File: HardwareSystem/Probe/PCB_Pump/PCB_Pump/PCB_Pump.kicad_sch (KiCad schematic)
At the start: 4 parts, among them Q1 IRF510

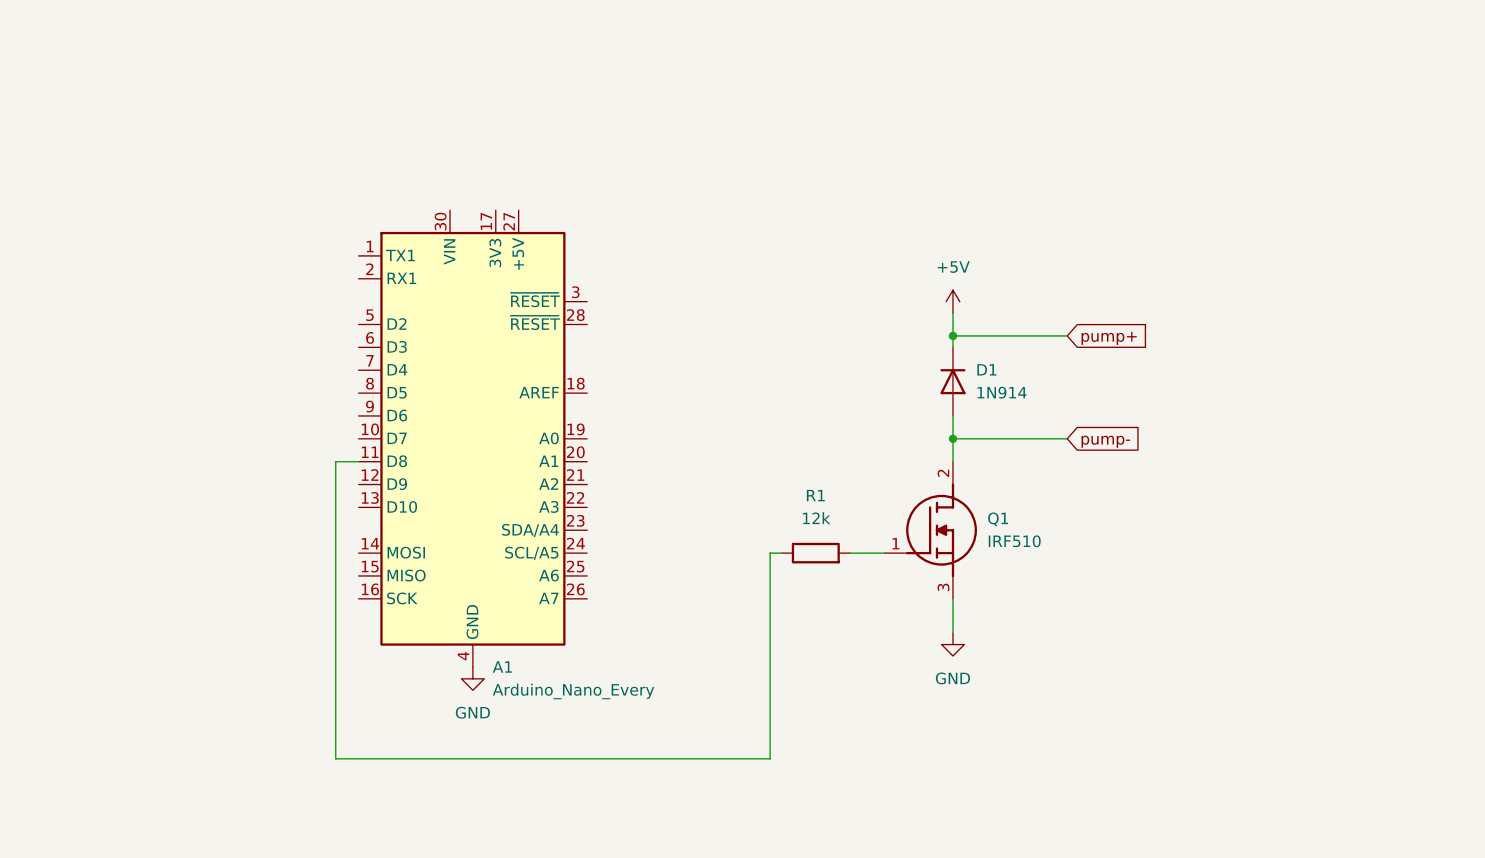
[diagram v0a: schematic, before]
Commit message: pump pcb work
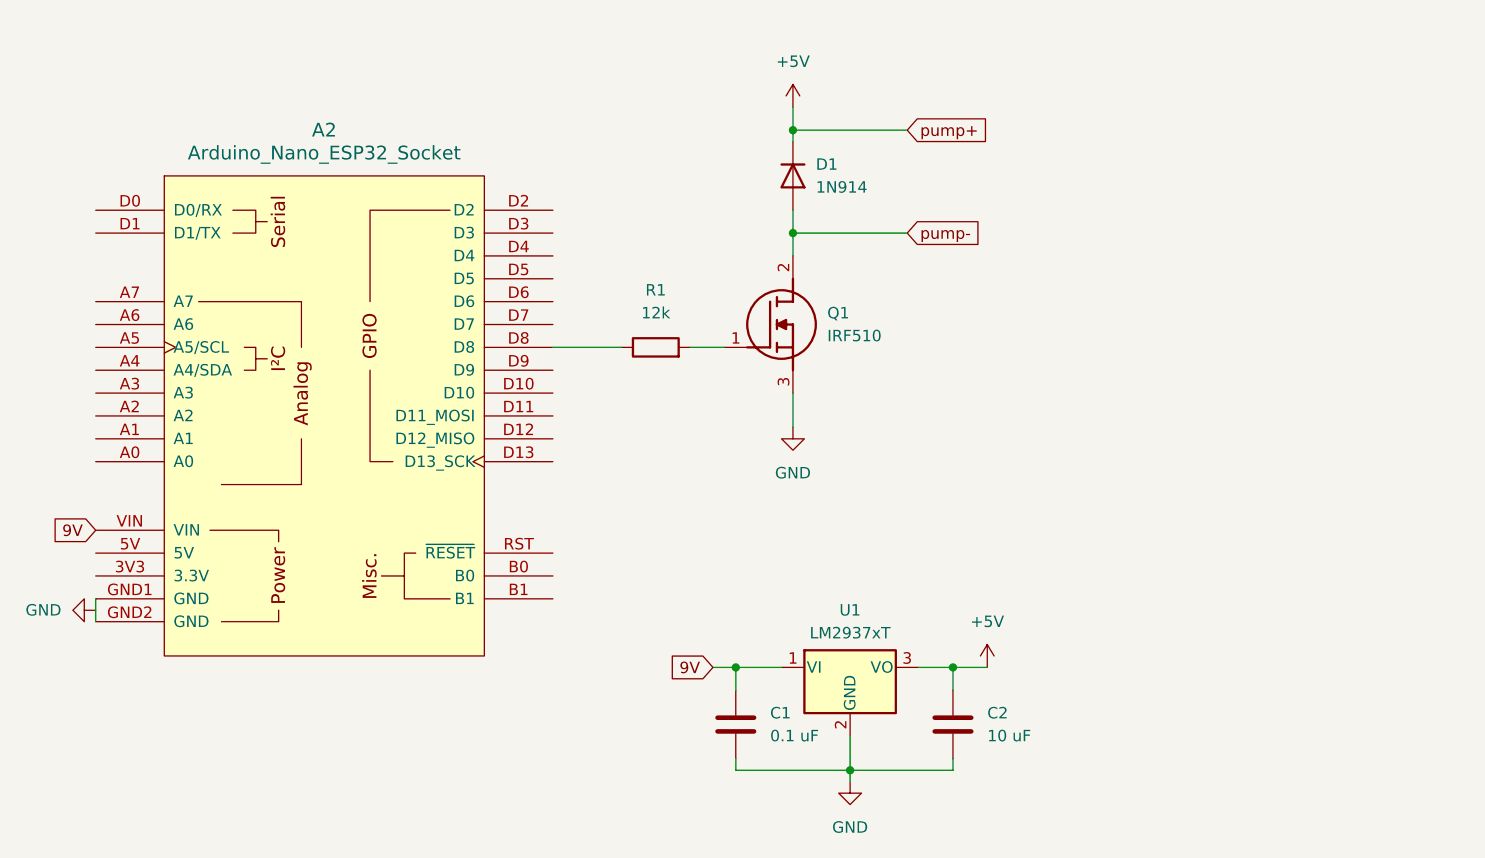
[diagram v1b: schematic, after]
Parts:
- removed A1: Arduino_Nano_Every, Module:Arduino_Nano, symbol MCU_Module:Arduino_Nano_Every
- added A2: Arduino_Nano_ESP32_Socket, footprints:Arduino_Nano_ESP32_Socket, symbol arduino-library:Arduino_Nano_ESP32_Socket
- added C1: 0.1 uF, Capacitor_THT:C_Axial_L3.8mm_D2.6mm_P7.50mm_Horizontal, symbol Device:C
- added C2: 10 uF, Capacitor_THT:C_Axial_L5.1mm_D3.1mm_P7.50mm_Horizontal, symbol Device:C
- added U1: LM2937xT, Package_TO_SOT_THT:TO-220-3_Vertical, symbol Regulator_Linear:LM2937xT
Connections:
- net +5V: now also C2.1, U1.3 (VO)
- net GND: now also C1.2, C2.2, U1.2 (GND)
- net at R1.1: now also A2.D8
- new net: A2.GND1 (GND), A2.GND2 (GND)
- new net 9V: A2.VIN, C1.1, U1.1 (VI)
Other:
- moved on the sheet: D1, Q1, R1

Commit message: finished PCB pump
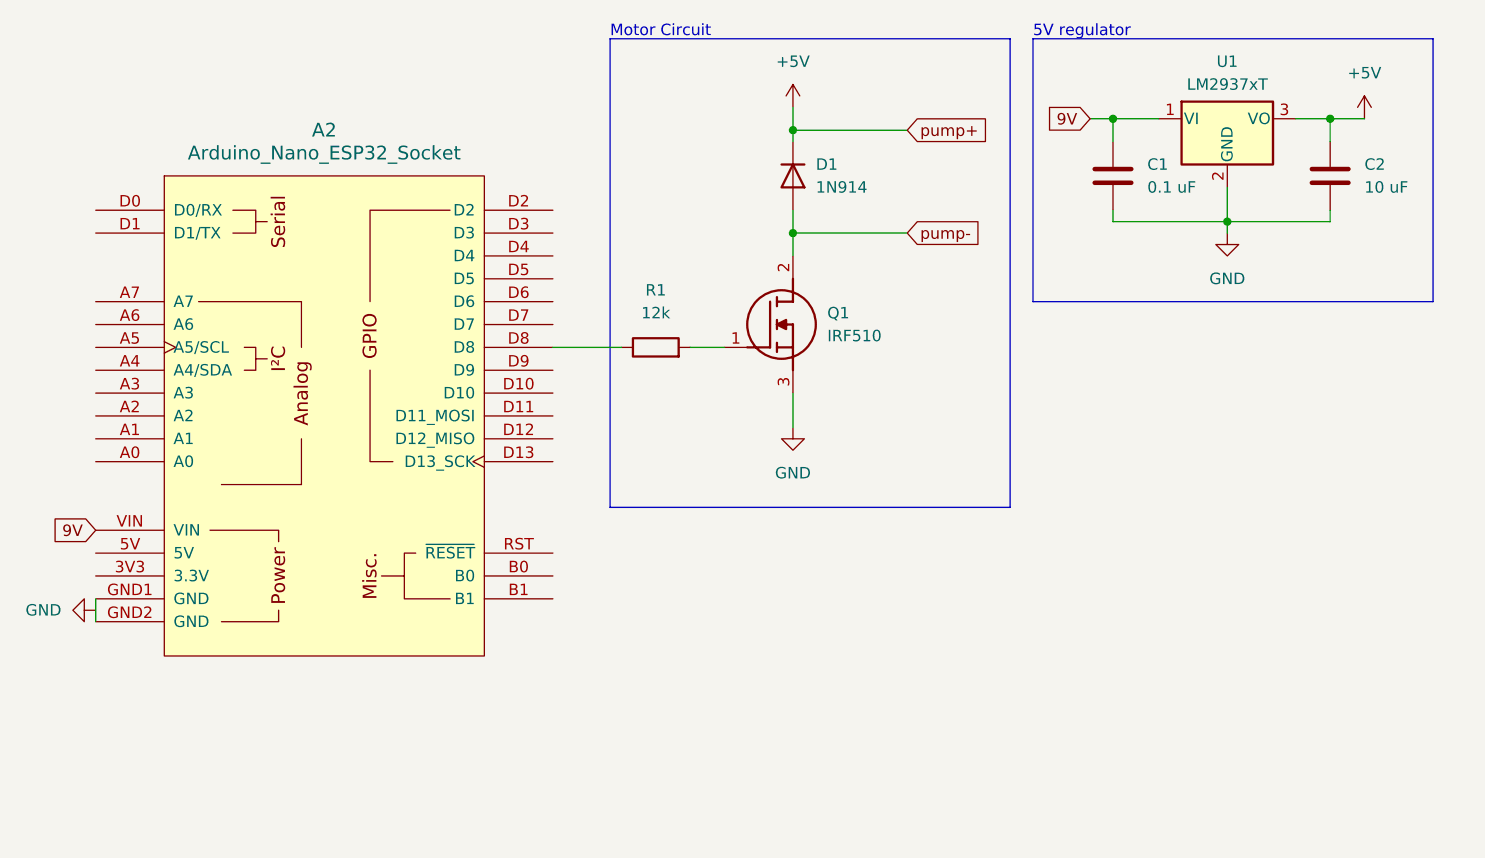
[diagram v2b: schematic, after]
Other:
- note added: "5V regulator"
- note added: "Motor Circuit"
- moved on the sheet: C1, C2, U1
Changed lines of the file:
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@@
 (kicad_sch (version 20230121) (generator eeschema)
   (paper "A4")
-  (junction (at 110.49 104.14) (diameter 0) (color 0 0 0 0)
-  )
-  (junction (at 121.92 92.71) (diameter 0) (color 0 0 0 0)
+  (junction (at 152.4 43.18) (diameter 0) (color 0 0 0 0)
+  )
+  (junction (at 163.83 31.75) (diameter 0) (color 0 0 0 0)
   )
   (junction (at 104.14 44.45) (diameter 0) (color 0 0 0 0)
@@
   (junction (at 104.14 33.02) (diameter 0) (color 0 0 0 0)
   )
-  (junction (at 97.79 92.71) (diameter 0) (color 0 0 0 0)
+  (junction (at 139.7 31.75) (diameter 0) (color 0 0 0 0)
   )
   (wire (pts (xy 104.14 62.23) (xy 104.14 66.04))
@@
     (stroke (width 0) (type default))
   )
-  (wire (pts (xy 95.25 92.71) (xy 97.79 92.71))
-    (stroke (width 0) (type default))
-  )
-  (wire (pts (xy 121.92 92.71) (xy 125.73 92.71))
+  (wire (pts (xy 137.16 31.75) (xy 139.7 31.75))
+    (stroke (width 0) (type default))
+  )
+  (wire (pts (xy 163.83 31.75) (xy 167.64 31.75))
     (stroke (width 0) (type default))
   )
@@
     (stroke (width 0) (type default))
   )
-  (wire (pts (xy 97.79 92.71) (xy 97.79 95.25))
-    (stroke (width 0) (type default))
-  )
-  (wire (pts (xy 110.49 104.14) (xy 121.92 104.14))
-    (stroke (width 0) (type default))
-  )
-  (wire (pts (xy 121.92 102.87) (xy 121.92 104.14))
-    (stroke (width 0) (type default))
-  )
-  (wire (pts (xy 97.79 104.14) (xy 110.49 104.14))
+  (wire (pts (xy 139.7 31.75) (xy 139.7 34.29))
+    (stroke (width 0) (type default))
+  )
+  (wire (pts (xy 152.4 43.18) (xy 163.83 43.18))
+    (stroke (width 0) (type default))
+  )
+  (wire (pts (xy 163.83 41.91) (xy 163.83 43.18))
+    (stroke (width 0) (type default))
+  )
+  (wire (pts (xy 139.7 43.18) (xy 152.4 43.18))
     (stroke (width 0) (type default))
   )
@@
     (stroke (width 0) (type default))
   )
-  (wire (pts (xy 121.92 92.71) (xy 121.92 95.25))
+  (wire (pts (xy 163.83 31.75) (xy 163.83 34.29))
     (stroke (width 0) (type default))
   )
@@
     (stroke (width 0) (type default))
   )
-  (wire (pts (xy 110.49 105.41) (xy 110.49 104.14))
+  (wire (pts (xy 152.4 44.45) (xy 152.4 43.18))
     (stroke (width 0) (type default))
   )
@@
     (stroke (width 0) (type default))
   )
-  (wire (pts (xy 110.49 104.14) (xy 110.49 100.33))
+  (wire (pts (xy 152.4 43.18) (xy 152.4 39.37))
     (stroke (width 0) (type default))
   )
@@
     (stroke (width 0) (type default))
   )
-  (wire (pts (xy 97.79 92.71) (xy 102.87 92.71))
-    (stroke (width 0) (type default))
-  )
-  (wire (pts (xy 97.79 102.87) (xy 97.79 104.14))
-    (stroke (width 0) (type default))
-  )
-  (wire (pts (xy 118.11 92.71) (xy 121.92 92.71))
-    (stroke (width 0) (type default))
-  )
-  (global_label "9V" (shape input) (at 95.25 92.71 180) (fields_autoplaced)
+  (wire (pts (xy 139.7 31.75) (xy 144.78 31.75))
+    (stroke (width 0) (type default))
+  )
+  (wire (pts (xy 139.7 41.91) (xy 139.7 43.18))
+    (stroke (width 0) (type default))
+  )
+  (wire (pts (xy 160.02 31.75) (xy 163.83 31.75))
+    (stroke (width 0) (type default))
+  )
+  (rectangle (start 130.81 22.86) (end 175.26 52.07)
+    (stroke (width 0) (type default))
+    (fill (type none))
+  )
+  (rectangle (start 83.82 22.86) (end 128.27 74.93)
+    (stroke (width 0) (type default))
+    (fill (type none))
+  )
+  (text "5V regulator" (at 130.81 22.86 0)
+    (effects (font (size 1.27 1.27)) (justify left bottom))
+  )
+  (text "Motor Circuit" (at 83.82 22.86 0)
+    (effects (font (size 1.27 1.27)) (justify left bottom))
+  )
+  (global_label "9V" (shape input) (at 137.16 31.75 180) (fields_autoplaced)
     (effects (font (size 1.27 1.27)) (justify right))
-    (property "Intersheetrefs" "${INTERSHEET_REFS}" (at 89.9667 92.71 0)
+    (property "Intersheetrefs" "${INTERSHEET_REFS}" (at 131.8767 31.75 0)
       (effects (font (size 1.27 1.27)) (justify right) hide)
     )
@@
     )
   )
-  (symbol (lib_id "power:GND") (at 110.49 105.41 0) (unit 1)
-    (in_bom yes) (on_board yes) (dnp no) (fields_autoplaced)
-    (property "Reference" "#PWR05" (at 110.49 111.76 0)
-      (effects (font (size 1.27 1.27)) hide)
-    )
-    (property "Value" "GND" (at 110.49 110.49 0)
-      (effects (font (size 1.27 1.27)))
-    )
-    (property "Footprint" "" (at 110.49 105.41 0)
-      (effects (font (size 1.27 1.27)) hide)
-    )
-    (property "Datasheet" "" (at 110.49 105.41 0)
+  (symbol (lib_id "power:GND") (at 152.4 44.45 0) (unit 1)
+    (in_bom yes) (on_board yes) (dnp no) (fields_autoplaced)
+    (property "Reference" "#PWR05" (at 152.4 50.8 0)
+      (effects (font (size 1.27 1.27)) hide)
+    )
+    (property "Value" "GND" (at 152.4 49.53 0)
+      (effects (font (size 1.27 1.27)))
+    )
+    (property "Footprint" "" (at 152.4 44.45 0)
+      (effects (font (size 1.27 1.27)) hide)
+    )
+    (property "Datasheet" "" (at 152.4 44.45 0)
       (effects (font (size 1.27 1.27)) hide)
     )
@@
     )
   )
-  (symbol (lib_id "Regulator_Linear:LM2937xT") (at 110.49 92.71 0) (unit 1)
-    (in_bom yes) (on_board yes) (dnp no) (fields_autoplaced)
-    (property "Reference" "U1" (at 110.49 86.36 0)
-      (effects (font (size 1.27 1.27)))
-    )
-    (property "Value" "LM2937xT" (at 110.49 88.9 0)
-      (effects (font (size 1.27 1.27)))
-    )
-    (property "Footprint" "Package_TO_SOT_THT:TO-220-3_Vertical" (at 110.49 86.995 0)
+  (symbol (lib_id "Regulator_Linear:LM2937xT") (at 152.4 31.75 0) (unit 1)
+    (in_bom yes) (on_board yes) (dnp no) (fields_autoplaced)
+    (property "Reference" "U1" (at 152.4 25.4 0)
+      (effects (font (size 1.27 1.27)))
+    )
+    (property "Value" "LM2937xT" (at 152.4 27.94 0)
+      (effects (font (size 1.27 1.27)))
+    )
+    (property "Footprint" "Package_TO_SOT_THT:TO-220-3_Vertical" (at 152.4 26.035 0)
       (effects (font (size 1.27 1.27) italic) hide)
     )
-    (property "Datasheet" "http://www.ti.com/lit/ds/symlink/lm2937.pdf" (at 110.49 93.98 0)
+    (property "Datasheet" "http://www.ti.com/lit/ds/symlink/lm2937.pdf" (at 152.4 33.02 0)
       (effects (font (size 1.27 1.27)) hide)
     )
@@
     )
   )
-  (symbol (lib_id "Device:C") (at 121.92 99.06 0) (unit 1)
-    (in_bom yes) (on_board yes) (dnp no) (fields_autoplaced)
-    (property "Reference" "C2" (at 125.73 97.79 0)
-      (effects (font (size 1.27 1.27)) (justify left))
-    )
-    (property "Value" "10 uF" (at 125.73 100.33 0)
-      (effects (font (size 1.27 1.27)) (justify left))
-    )
-    (property "Footprint" "Capacitor_THT:C_Axial_L5.1mm_D3.1mm_P7.50mm_Horizontal" (at 122.8852 102.87 0)
-      (effects (font (size 1.27 1.27)) hide)
-    )
-    (property "Datasheet" "~" (at 121.92 99.06 0)
+  (symbol (lib_id "Device:C") (at 163.83 38.1 0) (unit 1)
+    (in_bom yes) (on_board yes) (dnp no) (fields_autoplaced)
+    (property "Reference" "C2" (at 167.64 36.83 0)
+      (effects (font (size 1.27 1.27)) (justify left))
+    )
+    (property "Value" "10 uF" (at 167.64 39.37 0)
+      (effects (font (size 1.27 1.27)) (justify left))
+    )
+    (property "Footprint" "Capacitor_THT:C_Axial_L5.1mm_D3.1mm_P7.50mm_Horizontal" (at 164.7952 41.91 0)
+      (effects (font (size 1.27 1.27)) hide)
+    )
+    (property "Datasheet" "~" (at 163.83 38.1 0)
       (effects (font (size 1.27 1.27)) hide)
     )
@@
     )
   )
-  (symbol (lib_id "Device:C") (at 97.79 99.06 0) (unit 1)
-    (in_bom yes) (on_board yes) (dnp no) (fields_autoplaced)
-    (property "Reference" "C1" (at 101.6 97.79 0)
-      (effects (font (size 1.27 1.27)) (justify left))
-    )
-    (property "Value" "0.1 uF" (at 101.6 100.33 0)
-      (effects (font (size 1.27 1.27)) (justify left))
-    )
-    (property "Footprint" "Capacitor_THT:C_Axial_L3.8mm_D2.6mm_P7.50mm_Horizontal" (at 98.7552 102.87 0)
-      (effects (font (size 1.27 1.27)) hide)
-    )
-    (property "Datasheet" "~" (at 97.79 99.06 0)
+  (symbol (lib_id "Device:C") (at 139.7 38.1 0) (unit 1)
+    (in_bom yes) (on_board yes) (dnp no) (fields_autoplaced)
+    (property "Reference" "C1" (at 143.51 36.83 0)
+      (effects (font (size 1.27 1.27)) (justify left))
+    )
+    (property "Value" "0.1 uF" (at 143.51 39.37 0)
+      (effects (font (size 1.27 1.27)) (justify left))
+    )
+    (property "Footprint" "Capacitor_THT:C_Axial_L3.8mm_D2.6mm_P7.50mm_Horizontal" (at 140.6652 41.91 0)
+      (effects (font (size 1.27 1.27)) hide)
+    )
+    (property "Datasheet" "~" (at 139.7 38.1 0)
       (effects (font (size 1.27 1.27)) hide)
     )
@@
     )
   )
-  (symbol (lib_id "power:+5V") (at 125.73 92.71 0) (unit 1)
-    (in_bom yes) (on_board yes) (dnp no) (fields_autoplaced)
-    (property "Reference" "#PWR06" (at 125.73 96.52 0)
-      (effects (font (size 1.27 1.27)) hide)
-    )
-    (property "Value" "+5V" (at 125.73 87.63 0)
-      (effects (font (size 1.27 1.27)))
-    )
-    (property "Footprint" "" (at 125.73 92.71 0)
-      (effects (font (size 1.27 1.27)) hide)
-    )
-    (property "Datasheet" "" (at 125.73 92.71 0)
-      (effects (font (size 1.27 1.27)) hide)
-    )
+  (symbol (lib_id "power:+5V") (at 167.64 31.75 0) (unit 1)
+    (in_bom yes) (on_board yes) (dnp no) (fields_autoplaced)
+    (property "Reference" "#PWR06" (at 167.64 35.56 0)
+      (effects (font (size 1.27 1.27)) hide)
+    )
+    (property "Value" "+5V" (at 167.64 26.67 0)
+      (effects (font (size 1.27 1.27)))
+    )
+    (property "Footprint" "" (at 167.64 31.75 0)
+      (effects (font (size 1.27 1.27)) hide)
+    )
+    (property "Datasheet" "" (at 167.64 31.75 0)
+      (effects (font (size 1.27 1.27)) hide)
+    )

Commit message: pcb pump revision
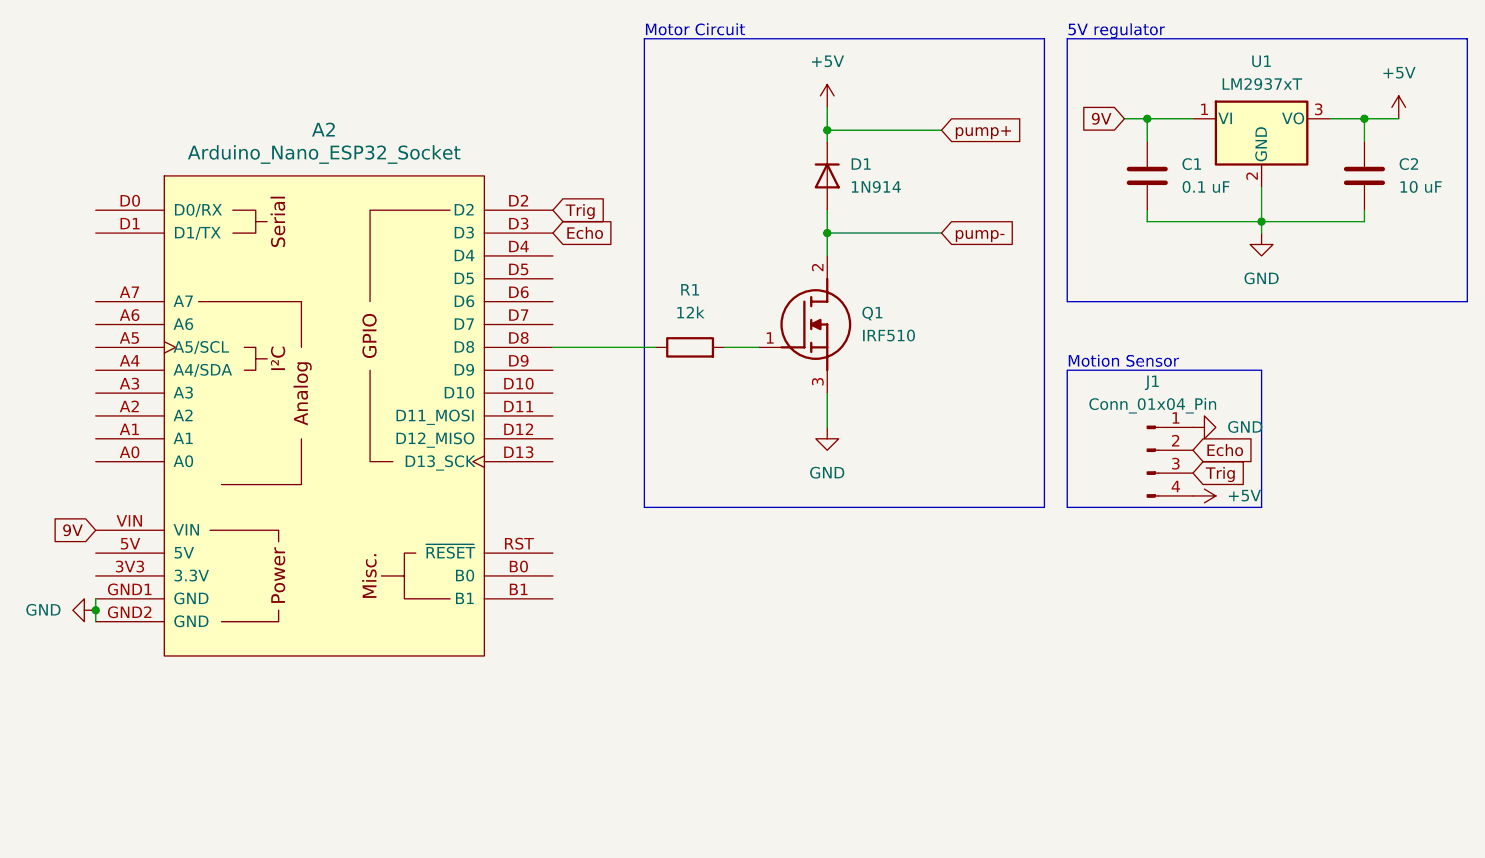
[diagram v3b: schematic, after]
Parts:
- added J1: Conn_01x04_Pin, Connector_PinHeader_2.54mm:PinHeader_1x04_P2.54mm_Vertical, symbol Connector:Conn_01x04_Pin
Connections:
- net +5V: now also J1.4 (Pin_4)
- net GND: now also A2.GND1 (GND), A2.GND2 (GND), J1.1 (Pin_1)
- net Trig: now reaches A2.D2
- net Trig: now also J1.3 (Pin_3)
- net Echo: now reaches A2.D3
- net Echo: now also J1.2 (Pin_2)
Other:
- note added: "Motion Sensor"
- moved on the sheet: C1, C2, D1, Q1, R1, U1
